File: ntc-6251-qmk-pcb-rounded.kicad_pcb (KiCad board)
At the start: 2 copper layers, 432 x 109.1 mm, 212 parts, among them J1 USB_B, U1 YAAJ_WeAct_BlackPill_Part_Lik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

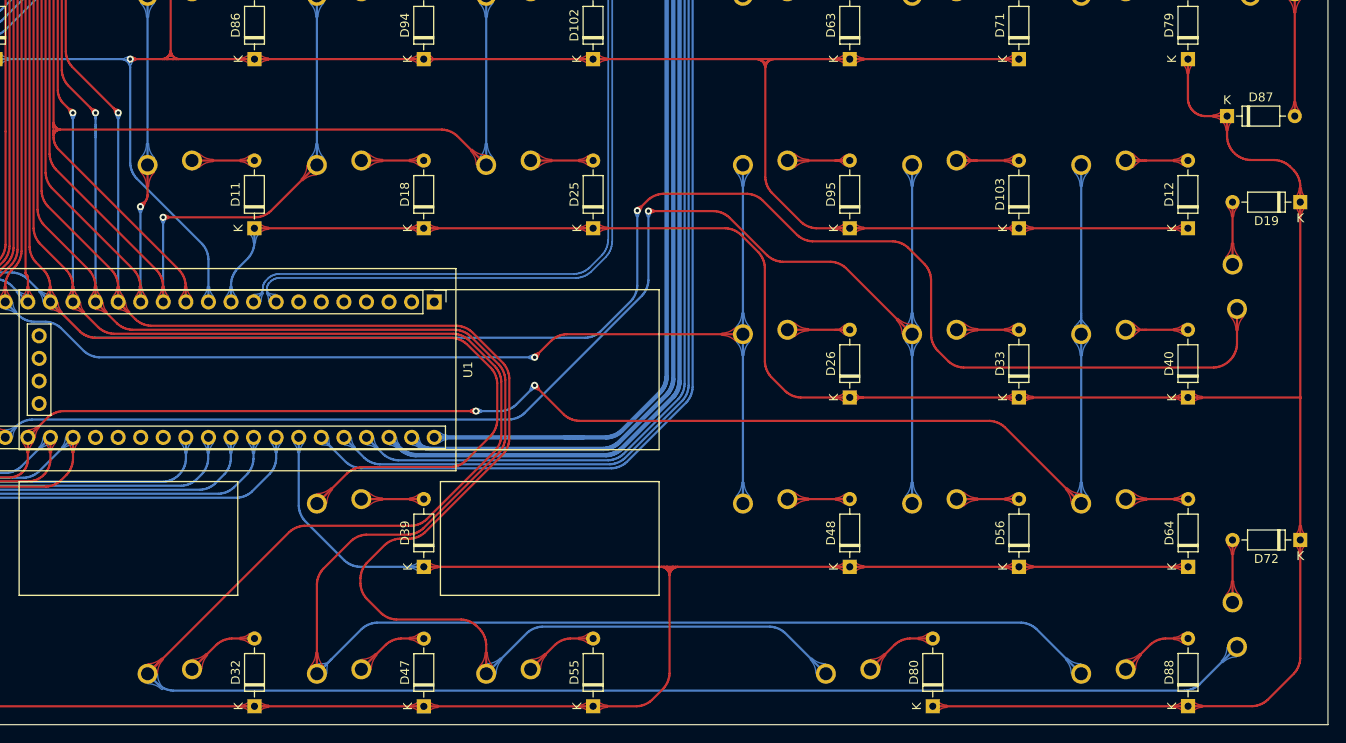
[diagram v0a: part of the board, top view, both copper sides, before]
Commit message: Small fixes to rounded pcb
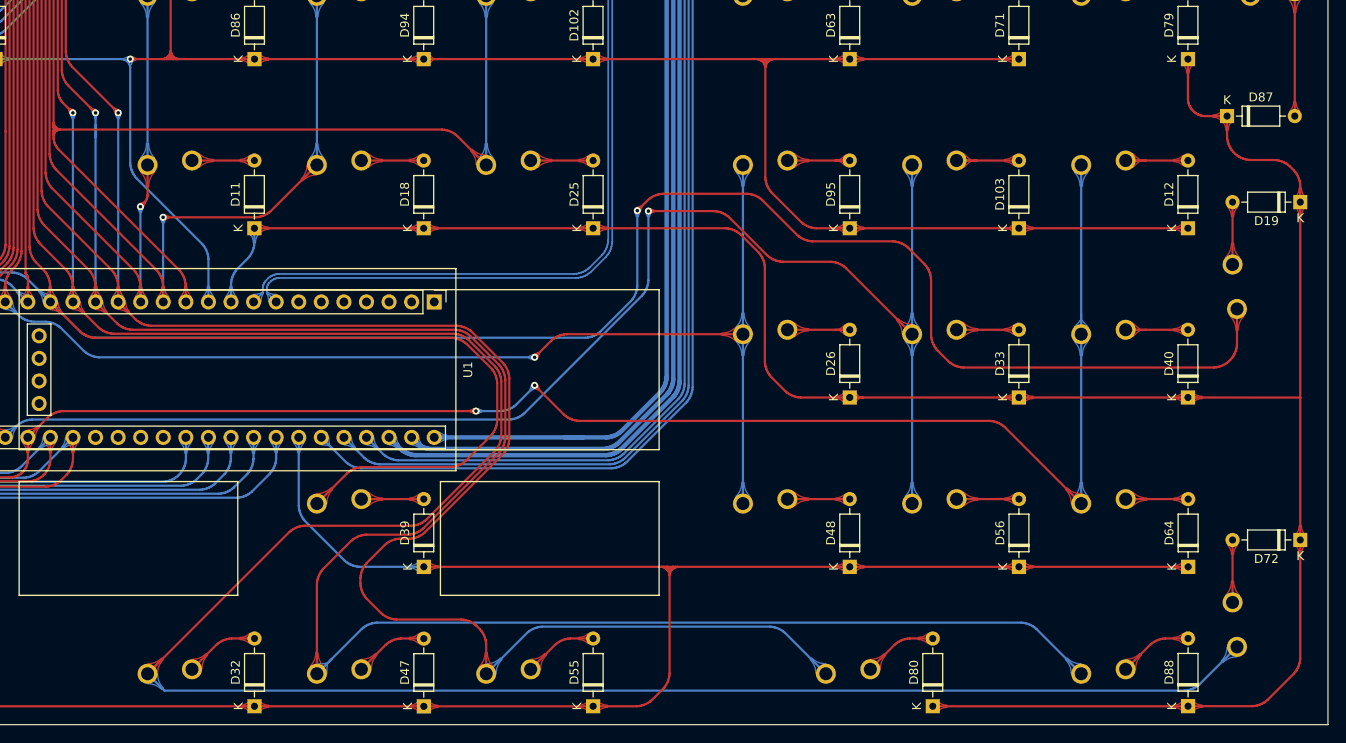
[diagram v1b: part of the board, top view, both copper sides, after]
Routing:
- net Row8: track 261.9 -> 262.5 mm
